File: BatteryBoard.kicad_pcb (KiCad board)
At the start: 4 copper layers, 13.7 x 10.4 mm, 20 parts, among them J1 Conn_01x05_Pin, J2 Conn_01x05_Pin, SW1 SW_SPST, U1 BQ25619ERTWR

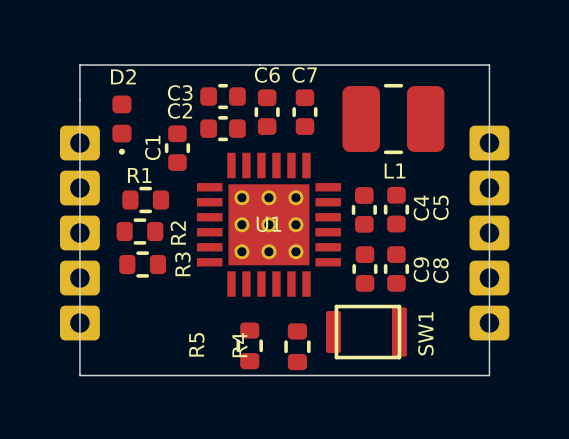
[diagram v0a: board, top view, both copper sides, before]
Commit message: Minor Update for Routing
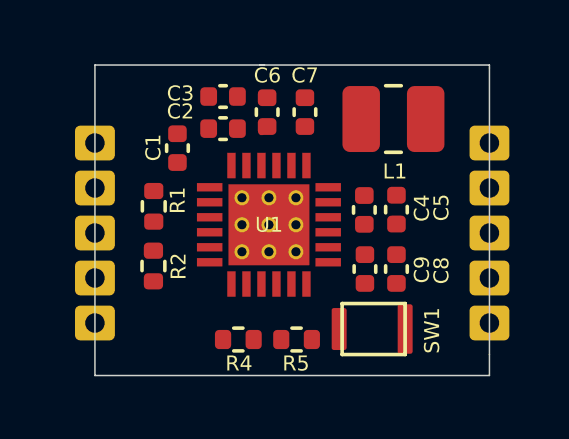
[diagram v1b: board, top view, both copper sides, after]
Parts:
- removed D2: LED, LED_SMD:LED_0402_1005Metric
- removed R3: 10k, Resistor_SMD:R_0402_1005Metric
- moved R4 1.98 mm to (72.4, 50.0), turned to 0 degrees
- moved R5 1.57 mm to (74.3, 50.0), turned to 0 degrees
- moved R2 1.23 mm to (69.5, 47.5), turned to -90 degrees
- moved J1 0.50 mm to (67.6, 43.4)
- moved R1 0.34 mm to (69.6, 45.5), turned to -90 degrees
- moved SW1 0.21 mm to (77.9, 49.6)
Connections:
- U1 pad 3: /PG -> unconnected-(U1-PMID_GOOD-Pad3)
- U1 pad 4: /STAT -> unconnected-(U1-STAT-Pad4)
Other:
- board size 13.7 x 10.4 mm -> 13.2 x 10.4 mm

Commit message: Out to Review
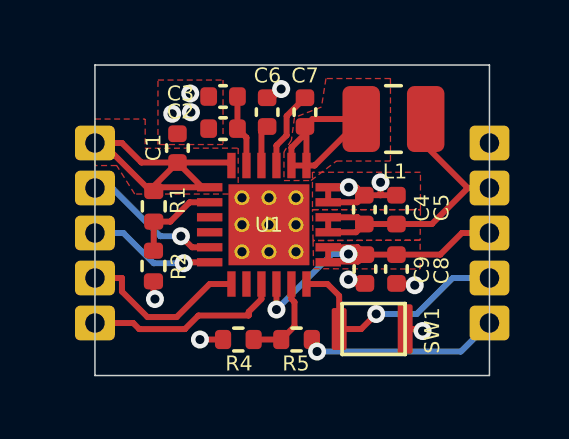
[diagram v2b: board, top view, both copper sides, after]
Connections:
- C7 pad 1: Net-(C7-Pad1) -> /SW
- J2 pad 4: Net-(J2-Pin_4) -> /BUTTON
- J2 pad 5: /SW -> /TS_BAT
- L1 pad 1: Net-(C7-Pad1) -> /SW
- R5 pad 2: Net-(J2-Pin_4) -> /TS_BAT
- SW1 pad 2: /SW -> /BUTTON
- U1 pad 12: /SW -> /BUTTON
- U1 pad 19: Net-(C7-Pad1) -> /SW
- U1 pad 20: Net-(C7-Pad1) -> /SW
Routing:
- net /VBAT: track 0.00 -> 12.2 mm, vias 0 -> 2
- net VBUS: track 0.00 -> 12.1 mm
- net /VSYS: track 0.00 -> 10.7 mm
- net GND: track 0.00 -> 8.44 mm, vias 0 -> 11
- net /BUTTON: track 0.00 -> 8.08 mm, vias 0 -> 1
- net /SW: track 0.00 -> 7.75 mm
- net /CE_N: track 0.00 -> 6.62 mm
- net /TS_BAT: track 0.00 -> 6.61 mm, vias 0 -> 1
- net /INT_N: track 0.00 -> 5.81 mm
- net /SCL: track 0.00 -> 4.64 mm, vias 0 -> 1
- net /SDA: track 0.00 -> 4.25 mm, vias 0 -> 1
- net /PSEL: track 0.00 -> 3.11 mm
- net /TS: track 0.00 -> 2.99 mm
- net Net-(U1-BTST): track 0.00 -> 2.65 mm
- net /PMID: track 0.00 -> 2.42 mm
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- added copper zone on F.Cu, net /SW
- added copper zone on F.Cu, net /VBAT
- added copper zone on F.Cu, net /VSYS
- added copper zone on F.Cu, net GND
- added copper zone on In1.Cu, net GND
- added copper zone on In2.Cu, net GND
- added copper zone on F.Cu, net VBUS
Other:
- outline, holes or cut-outs redrawn
